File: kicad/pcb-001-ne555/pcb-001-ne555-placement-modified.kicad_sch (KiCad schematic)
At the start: 14 parts, among them J1 +5 V / GND power input, U1 NE555D

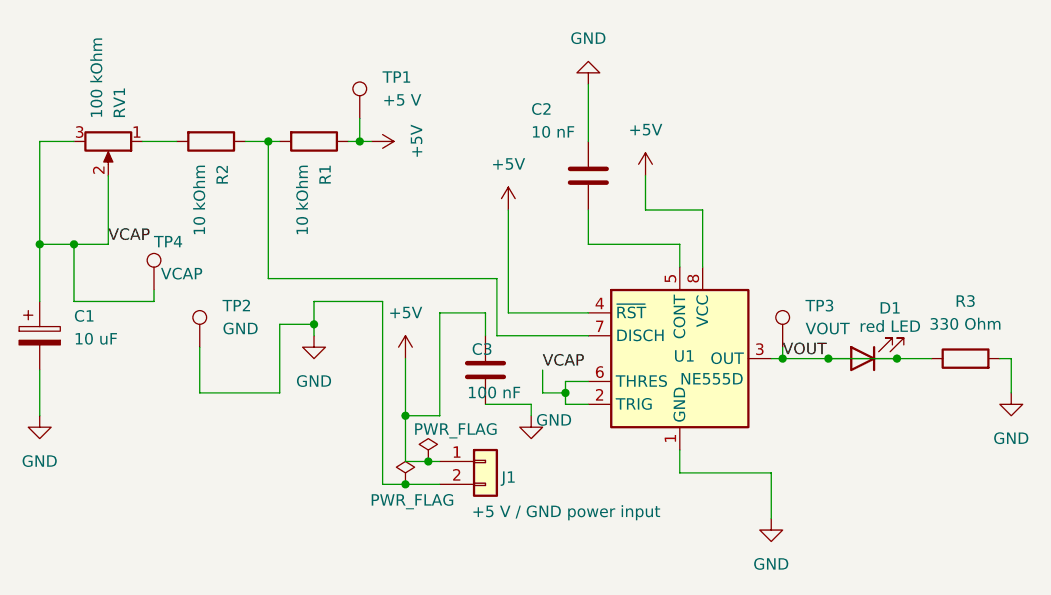
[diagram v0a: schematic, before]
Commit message: Update project files 2026-08-16 14:48:06
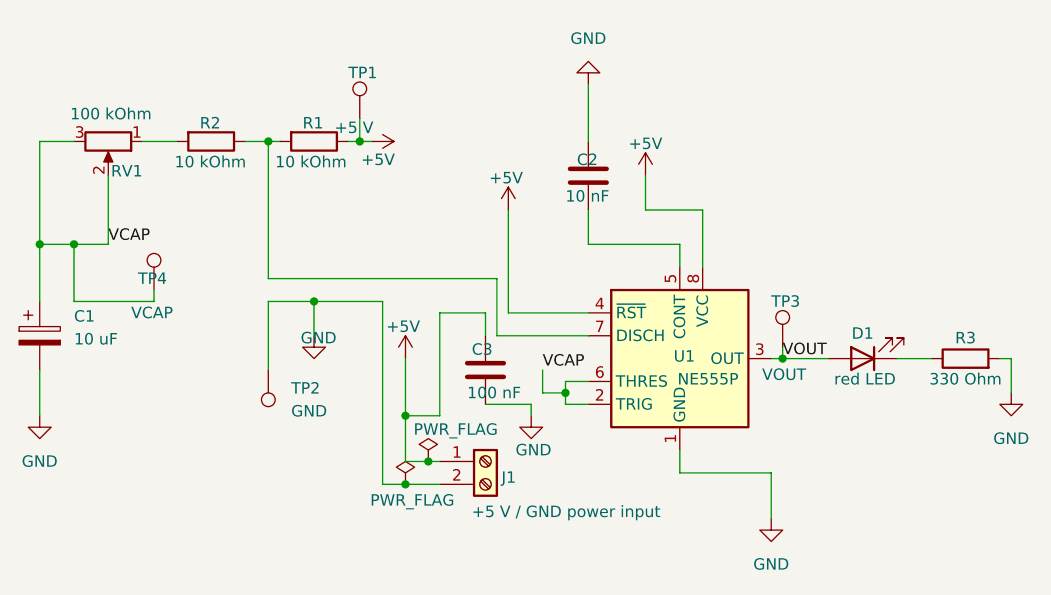
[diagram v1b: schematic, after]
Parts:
- J1: symbol Connector_Generic:Conn_01x02 -> Connector:Screw_Terminal_01x02
- U1: value NE555D -> NE555P; symbol Timer:NE555D -> Timer:NE555P
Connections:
- net VOUT: no longer D1.1 (K), R3.1
- new net: D1.1 (K), R3.1
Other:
- moved on the sheet: TP2
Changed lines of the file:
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@@
-	)
-	(junction
-		(at 194.31 102.87)
-		(diameter 0)
-		(color 0 0 0 0)
 	)
 	(junction
@@
 	)
 	(junction
-		(at 181.61 102.87)
+		(at 129.54 96.52)
 		(diameter 0)
 		(color 0 0 0 0)
@@
 	)
 	(junction
-		(at 186.69 102.87)
+		(at 181.61 102.87)
 		(diameter 0)
 		(color 0 0 0 0)
 	)
-	(junction
-		(at 129.54 99.06)
-		(diameter 0)
-		(color 0 0 0 0)
-	)
 	(wire
 		(pts
@@
 	(wire
 		(pts
-			(xy 125.73 99.06) (xy 129.54 99.06)
+			(xy 124.46 96.52) (xy 129.54 96.52)
 		)
 		(stroke
@@
 	(wire
 		(pts
-			(xy 116.84 101.6) (xy 116.84 106.68)
-		)
-		(stroke
-			(width 0)
-			(type default)
-		)
-	)
-	(wire
-		(pts
-			(xy 125.73 106.68) (xy 125.73 99.06)
-		)
-		(stroke
-			(width 0)
-			(type default)
-		)
-	)
-	(wire
-		(pts
 			(xy 157.48 107.95) (xy 160.02 107.95)
 		)
@@
 	(wire
 		(pts
-			(xy 116.84 106.68) (xy 125.73 106.68)
-		)
-		(stroke
-			(width 0)
-			(type default)
-		)
-	)
-	(wire
-		(pts
 			(xy 139.7 116.84) (xy 143.51 116.84)
 		)
@@
 	(wire
 		(pts
-			(xy 129.54 96.52) (xy 129.54 99.06)
+			(xy 129.54 96.52) (xy 129.54 100.33)
 		)
 		(stroke
@@
 	(wire
 		(pts
-			(xy 186.69 102.87) (xy 194.31 102.87)
-		)
-		(stroke
-			(width 0)
-			(type default)
-		)
-	)
-	(wire
-		(pts
 			(xy 102.87 90.17) (xy 106.68 90.17)
 		)
@@
 	(wire
 		(pts
-			(xy 129.54 99.06) (xy 129.54 100.33)
-		)
-		(stroke
-			(width 0)
-			(type default)
-		)
-	)
-	(wire
-		(pts
 			(xy 148.59 100.33) (xy 148.59 97.79)
 		)
@@
 		(pts
 			(xy 205.74 102.87) (xy 207.01 102.87)
+		)
+		(stroke
+			(width 0)
+			(type default)
+		)
+	)
+	(wire
+		(pts
+			(xy 124.46 96.52) (xy 124.46 104.14)
 		)
 		(stroke
@@
 		(in_pos_files yes)
 		(dnp no)
-		(fields_autoplaced yes)
 		(property "Reference" "#PWR04"
 			(at 139.7 106.68 0)
@@
 		)
 		(property "Value" "+5V"
-			(at 139.7 97.79 0)
+			(at 139.446 99.314 0)
 			(show_name no)
 			(do_not_autoplace no)
@@
 	)
 	(symbol
-		(lib_id "Timer:NE555D")
+		(lib_id "Timer:NE555P")
 		(at 170.18 102.87 0)
 		(unit 1)
@@
 			)
 		)
-		(property "Value" "NE555D"
-			(at 173.736 105.156 0)
-			(show_name no)
-			(do_not_autoplace no)
-			(effects
-				(font
-					(size 1.27 1.27)
-				)
+		(property "Value" "NE555P"
+			(at 169.926 105.156 0)
+			(show_name no)
+			(do_not_autoplace no)
+			(effects
+				(font
+					(size 1.27 1.27)
+				)
+				(justify left)
 			)
 		)
@@
 			)
 		)
-		(property "Description" "Precision Timers, 555 compatible, SOIC-8"
+		(property "Description" "Precision Timers, 555 compatible, PDIP-8"
 			(at 170.18 124.46 0)
 			(hide yes)
@@
 		(in_pos_files yes)
 		(dnp no)
-		(fields_autoplaced yes)
 		(property "Reference" "TP1"
-			(at 137.16 71.6279 0)
+			(at 133.35 71.12 0)
 			(show_name no)
 			(do_not_autoplace no)
@@
 		)
 		(property "Value" "+5 V"
-			(at 137.16 74.1679 0)
+			(at 131.826 77.216 0)
 			(show_name no)
 			(do_not_autoplace no)
@@
 		(dnp no)
 		(property "Reference" "C2"
-			(at 153.67 75.184 0)
+			(at 158.75 80.772 0)
 			(show_name no)
 			(do_not_autoplace no)
@@
 		)
 		(property "Value" "10 nF"
-			(at 153.67 77.724 0)
+			(at 157.48 84.836 0)
 			(show_name no)
 			(do_not_autoplace no)
@@
 		(in_pos_files yes)
 		(dnp no)
-		(fields_autoplaced yes)
 		(property "Reference" "R2"
-			(at 119.3801 81.28 0)
+			(at 116.84 76.708 90)
 			(show_name no)
 			(do_not_autoplace no)
@@
 		)
 		(property "Value" "10 kOhm"
-			(at 116.8401 81.28 0)
+			(at 114.046 81.026 90)
 			(show_name no)
 			(do_not_autoplace no)
@@
 		(in_pos_files yes)
 		(dnp no)
-		(fields_autoplaced yes)
 		(property "Reference" "R1"
-			(at 130.8101 81.28 0)
+			(at 128.27 76.708 90)
 			(show_name no)
 			(do_not_autoplace no)
@@
 		)
 		(property "Value" "10 kOhm"
-			(at 128.2701 81.28 0)
+			(at 125.222 81.026 90)
 			(show_name no)
 			(do_not_autoplace no)
@@
 		(in_pos_files yes)
 		(dnp no)
-		(fields_autoplaced yes)
 		(property "Reference" "TP3"
-			(at 184.15 97.0279 0)
+			(at 180.34 96.52 0)
 			(show_name no)
 			(do_not_autoplace no)
@@
 		)
 		(property "Value" "VOUT"
-			(at 184.15 99.5679 0)
+			(at 179.324 104.648 0)
 			(show_name no)
 			(do_not_autoplace no)
@@
 		(in_pos_files yes)
 		(dnp no)
-		(fields_autoplaced yes)
 		(property "Reference" "R3"
-			(at 201.93 96.52 90)
+			(at 201.93 100.584 90)
 			(show_name no)
 			(do_not_autoplace no)
@@
 		)
 		(property "Value" "330 Ohm"
-			(at 201.93 99.06 90)
+			(at 201.93 105.156 90)
 			(show_name no)
 			(do_not_autoplace no)
@@
 	(symbol
 		(lib_id "Connector:TestPoint")
-		(at 116.84 101.6 0)
+		(at 124.46 104.14 180)
 		(unit 1)
 		(body_style 1)
@@
 		(fields_autoplaced yes)
 		(property "Reference" "TP2"
-			(at 119.38 97.0279 0)
-			(show_name no)
-			(do_not_autoplace no)
-			(effects
-				(font
-					(size 1.27 1.27)
-				)
-				(justify left)
+			(at 127 106.1719 0)
+			(show_name no)
+			(do_not_autoplace no)
+			(effects
+				(font
+					(size 1.27 1.27)
+				)
+				(justify right)
 			)
 		)
 		(property "Value" "GND"
-			(at 119.38 99.5679 0)
-			(show_name no)
-			(do_not_autoplace no)
-			(effects
-				(font
-					(size 1.27 1.27)
-				)
-				(justify left)
+			(at 127 108.7119 0)
+			(show_name no)
+			(do_not_autoplace no)
+			(effects
+				(font
+					(size 1.27 1.27)
+				)
+				(justify right)
 			)
 		)
 		(property "Footprint" "TestPoint:TestPoint_THTPad_D2.0mm_Drill1.0mm"
-			(at 121.92 101.6 0)
+			(at 119.38 104.14 0)
 			(hide yes)
 			(show_name no)
@@
 		)
 		(property "Datasheet" ""
-			(at 121.92 101.6 0)
+			(at 119.38 104.14 0)
 			(hide yes)
 			(show_name no)
@@
 		)
 		(property "Description" "test point"
-			(at 116.84 101.6 0)
+			(at 124.46 104.14 0)
 			(hide yes)
 			(show_name no)
@@
 		(in_pos_files yes)
 		(dnp no)
-		(fields_autoplaced yes)
 		(property "Reference" "#PWR02"
 			(at 129.54 106.68 0)
@@
 		)
 		(property "Value" "GND"
-			(at 129.54 105.41 0)
+			(at 130.048 100.584 0)
 			(show_name no)
 			(do_not_autoplace no)
@@
 		(in_pos_files yes)
 		(dnp no)
-		(fields_autoplaced yes)
 		(property "Reference" "RV1"
-			(at 107.9501 76.2 0)
+			(at 110.49 82.042 90)
 			(show_name no)
 			(do_not_autoplace no)
@@
 		)
 		(property "Value" "100 kOhm"
-			(at 105.4101 76.2 0)
+			(at 111.506 75.692 90)
 			(show_name no)
 			(do_not_autoplace no)
@@
 		(dnp no)
 		(property "Reference" "TP4"
-			(at 111.76 89.916 0)
+			(at 109.982 93.98 0)
 			(show_name no)
 			(do_not_autoplace no)
@@
 		)
 		(property "Value" "VCAP"
-			(at 112.522 93.472 0)
+			(at 109.22 97.79 0)
 			(show_name no)
 			(do_not_autoplace no)
@@
 		(in_pos_files yes)
 		(dnp no)
-		(fields_autoplaced yes)
 		(property "Reference" "#PWR08"
 			(at 132.08 78.74 0)
@@
 		)
 		(property "Value" "+5V"
-			(at 140.97 78.74 0)
+			(at 136.652 80.772 90)
 			(show_name no)
 			(do_not_autoplace no)
@@
 		)
 		(property "Value" "GND"
-			(at 156.21 109.728 0)
+			(at 153.924 113.03 0)
 			(show_name no)
 			(do_not_autoplace no)
@@
 		(dnp no)
 		(property "Reference" "D1"
-			(at 193.548 97.282 0)
+			(at 190.5 100.076 0)
 			(show_name no)
 			(do_not_autoplace no)
@@
 		)
 		(property "Value" "red LED"
-			(at 193.548 99.314 0)
+			(at 190.754 105.156 0)
 			(show_name no)
 			(do_not_autoplace no)
@@
 		(in_pos_files yes)
 		(dnp no)
-		(fields_autoplaced yes)
 		(property "Reference" "#PWR03"
 			(at 151.13 90.17 0)
@@
 		)
 		(property "Value" "+5V"
-			(at 151.13 81.28 0)
+			(at 150.876 82.804 0)
 			(show_name no)
 			(do_not_autoplace no)
@@
 		(in_pos_files yes)
 		(dnp no)
-		(fields_autoplaced yes)
 		(property "Reference" "#PWR01"
 			(at 166.37 86.36 0)
@@
 		)
 		(property "Value" "+5V"
-			(at 166.37 77.47 0)
+			(at 166.37 78.994 0)
 			(show_name no)
 			(do_not_autoplace no)
@@
 	)
 	(symbol
-		(lib_id "Connector_Generic:Conn_01x02")
+		(lib_id "Connector:Screw_Terminal_01x02")
 		(at 148.59 114.3 0)
 		(unit 1)
@@
 			)
 		)
-		(property "Description" "Generic connector, single row, 01x02, script generated (kicad-library-utils/schlib/autogen/connector/)"
+		(property "Description" "Generic screw terminal, single row, 01x02, script generated (kicad-library-utils/schlib/autogen/connector/)"
 			(at 148.59 114.3 0)
 			(hide yes)
